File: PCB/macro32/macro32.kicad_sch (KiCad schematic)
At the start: 14 parts, among them J1 OLED, J2 OLED, J3 Magnetic connector, J4 Magnetic connector, J5 Magnetic connector, J6 Magnetic connector, SW1 RST, U1 SuperMini_NRF52840

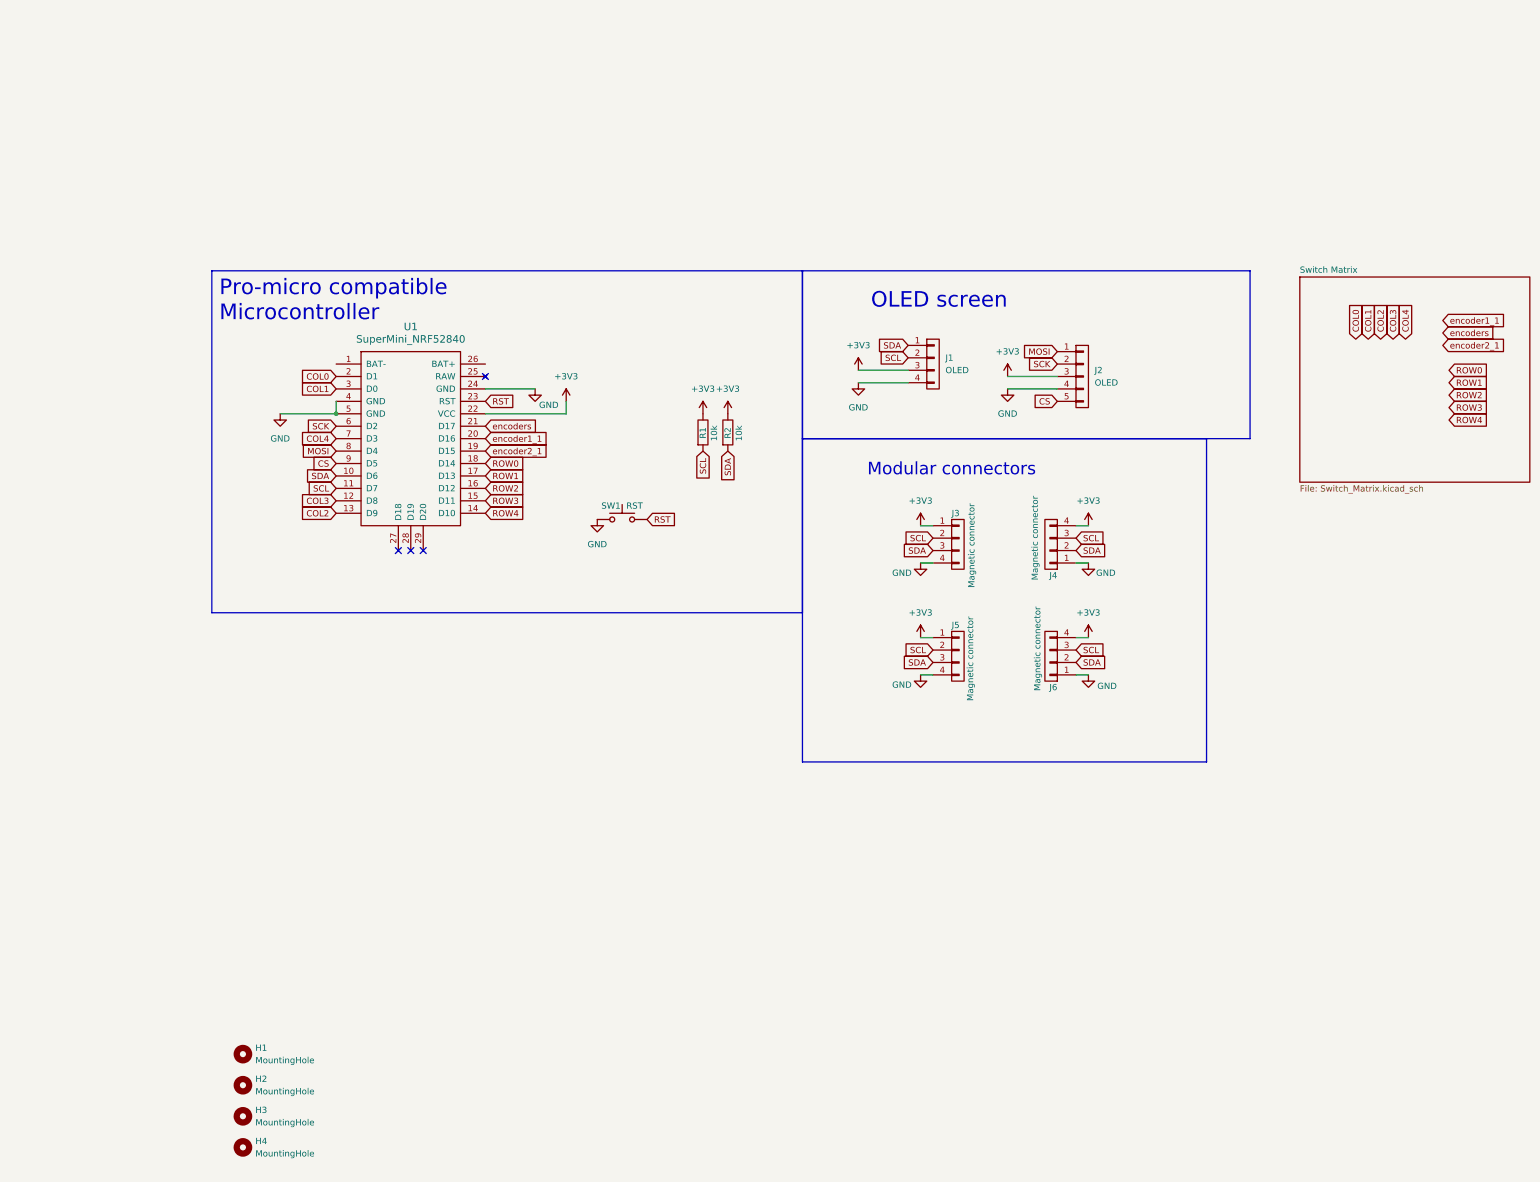
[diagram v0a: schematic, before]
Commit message: macro32_v2_schem&pcb
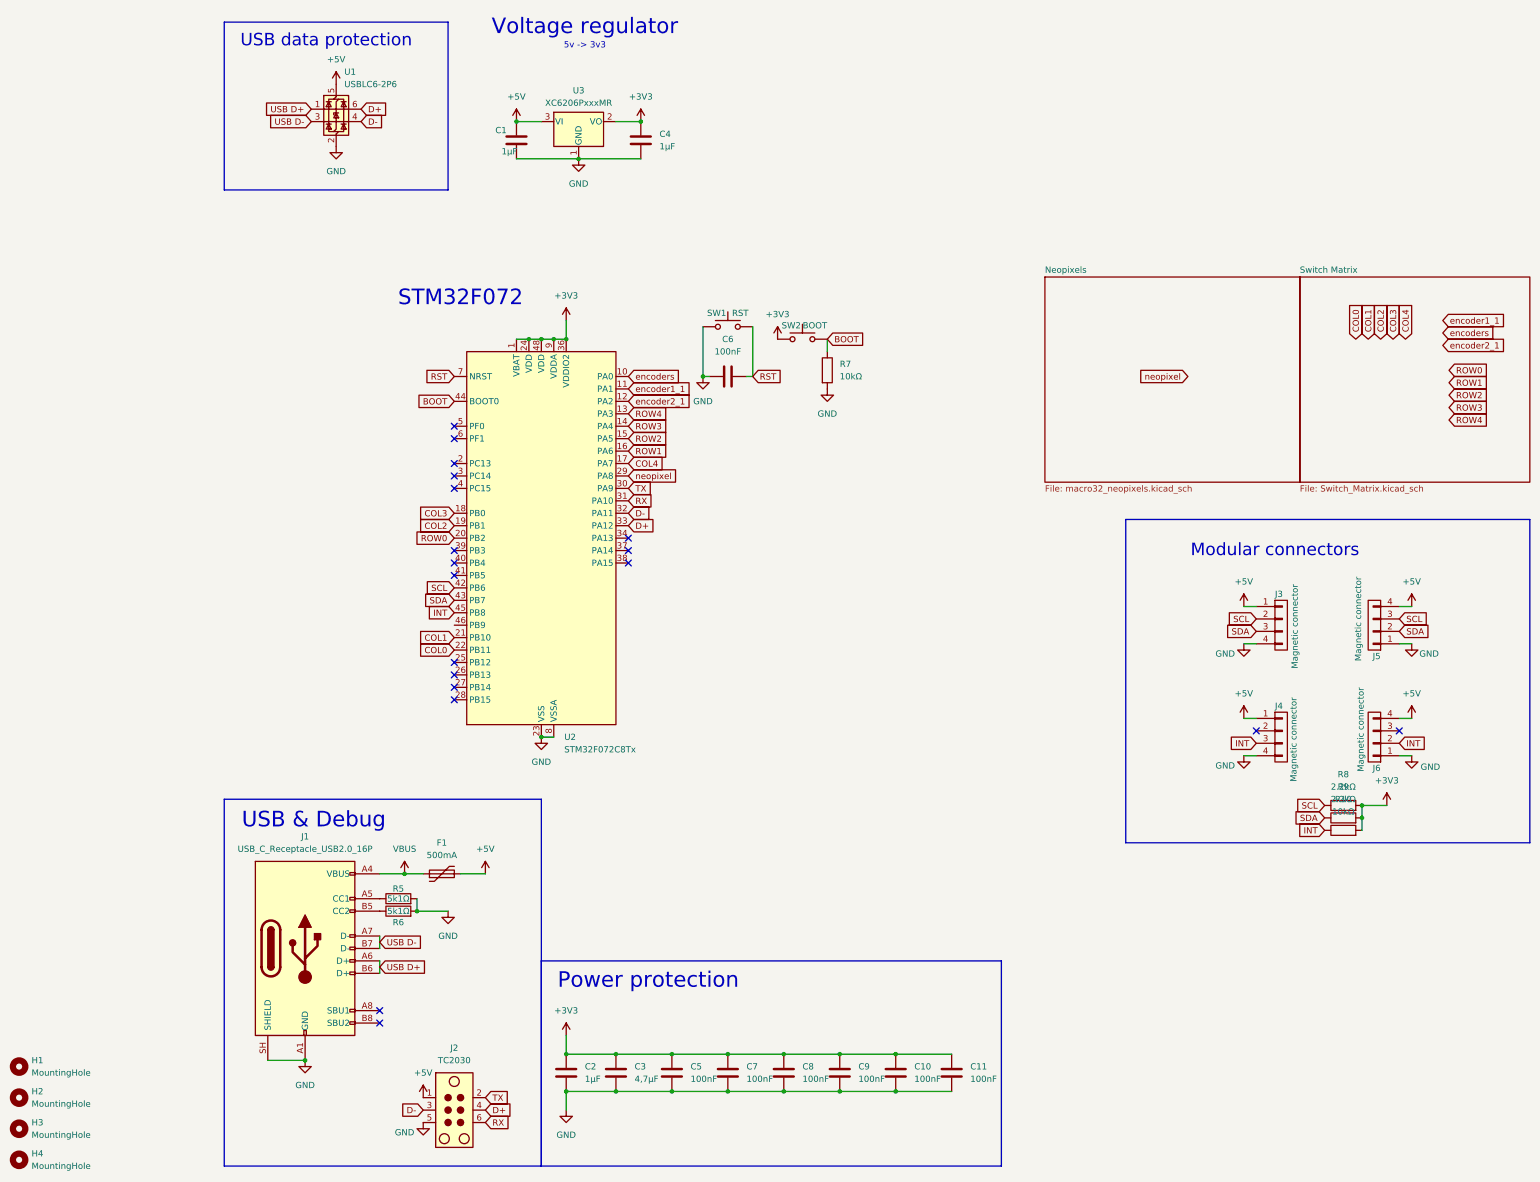
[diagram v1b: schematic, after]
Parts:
- removed J1: OLED, KillrOfLife_Connectors:OLED_4Pin, symbol KillrOfLife:OLED-4pin
- removed J2: OLED, KillrOfLife_Connectors:OLED_5Pin, symbol KillrOfLife:OLED-5pin
- removed R1, R2: 10k, Resistor_SMD:R_0805_2012Metric_Pad1.20x1.40mm_HandSolder, symbol Device:R
- removed U1: SuperMini_NRF52840, KillrOfLife_MCU:SuperMini_NRF52850_pro_micro, symbol ScottoKeebs:MCU_SuperMini_NRF52840
- added C1, C2, C4: 1μF, Capacitor_SMD:C_0805_2012Metric_Pad1.18x1.45mm_HandSolder, symbol Device:C
- added C10, C11, C5, C6, C7, C8, C9: 100nF, Capacitor_SMD:C_0805_2012Metric_Pad1.18x1.45mm_HandSolder, symbol Device:C
- added C3: 4,7μF, Capacitor_SMD:C_0805_2012Metric_Pad1.18x1.45mm_HandSolder, symbol Device:C
- added F1: 500mA, KillrOfLife_Components:Resistor_1206, symbol Device:Polyfuse
- added J1: USB_C_Receptacle_USB2.0_16P, Connector_USB:USB_C_Receptacle_GCT_USB4110, symbol Connector:USB_C_Receptacle_USB2.0_16P
- added J2: TC2030, Connector:Tag-Connect_TC2030-IDC-FP_2x03_P1.27mm_Vertical, symbol Connector:TC2030
- added R10, R7: 10kΩ, KillrOfLife_Components:Resistor_0805, symbol Device:R
- added R5, R6: 5k1Ω, KillrOfLife_Components:Resistor_0805, symbol Device:R
- added R8, R9: 2.2kΩ, KillrOfLife_Components:Resistor_0805, symbol Device:R
- added SW2: BOOT, Button_Switch_SMD:SW_SPST_TS-1088-xR020, symbol Switch:SW_Push
- added U1: USBLC6-2P6, Package_TO_SOT_SMD:SOT-666, symbol Power_Protection:USBLC6-2P6
- added U2: STM32F072C8Tx, Package_QFP:LQFP-48_7x7mm_P0.5mm, symbol MCU_ST_STM32F0:STM32F072C8Tx
- added U3: XC6206PxxxMR, Package_TO_SOT_SMD:SOT-23-3, symbol Regulator_Linear:XC6206PxxxMR
- J3: footprint Library:fakemag4pin90degFemale -> KillrOfLife_Connectors:fakemag4pin90degFemale
- J4: renamed from J5; footprint Library:fakemag4pin90degFemale -> KillrOfLife_Connectors:fakemag4pin90degFemale
- J5: renamed from J4; footprint Library:fakemag4pin90degMale -> KillrOfLife_Connectors:fakemag4pin90degFemale
- J6: footprint Library:fakemag4pin90degMale -> KillrOfLife_Connectors:fakemag4pin90degFemale
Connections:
- net +3V3: now also C10.1, C11.1, C2.1, C3.1, C4.1, C5.1, C7.1, C8.1, C9.1, R10.2, R8.2, R9.2, SW2.1, U2.1 (VBAT), U2.24 (VDD), U2.36 (VDDIO2), U2.48 (VDD), U2.9 (VDDA), U3.2 (VO); no longer J3.1 (P1), J4.1 (P1), J5.4 (P4), J6.4 (P4)
- net COL0: now also U2.22 (PB11)
- net COL1: now also U2.21 (PB10)
- net COL2: now also U2.19 (PB1)
- net COL3: now also U2.18 (PB0)
- net COL4: now also U2.17 (PA7)
- net GND: now also C1.2, C10.2, C11.2, C2.2, C3.2, C4.2, C5.2, C6.1, C7.2, C8.2, C9.2, J1.A1 (GND), J1.A12 (GND), J1.B1 (GND), J1.B12 (GND), J1.SH (SHIELD), J2.5, R5.2, R6.2, R7.2, U1.2 (GND), U2.23 (VSS), U2.35 (VSS), U2.47 (VSS), U2.8 (VSSA), U3.1 (GND)
- net ROW0: now also U2.20 (PB2)
- net ROW1: now also U2.16 (PA6)
- net ROW2: now also U2.15 (PA5)
- net ROW3: now also U2.14 (PA4)
- net ROW4: now also U2.13 (PA3)
- net RST: now also C6.2, U2.7 (NRST)
- net SCL: now also R8.1, U2.42 (PB6); no longer J4.2 (P2), J6.3 (P3)
- net SDA: now also R9.1, U2.43 (PB7); no longer J4.3 (P3), J6.2 (P2)
- net encoder1_1: now also U2.11 (PA1)
- net encoder2_1: now also U2.12 (PA2)
- net encoders: now also U2.10 (PA0)
- new net: J1.B5 (CC2), R6.1
- new net: J1.A5 (CC1), R5.1
- new net +5V: C1.1, F1.2, J2.1, J3.1 (P1), J4.1 (P1), J5.4 (P4), J6.4 (P4), U1.5 (VBUS), U3.3 (VI)
- new net BOOT: R7.1, SW2.2, U2.44 (BOOT0)
- new net D+: J2.4, U1.6 (I/O1), U2.33 (PA12)
- new net D-: J2.3, U1.4 (I/O2), U2.32 (PA11)
- new net INT: J4.3 (P3), J6.2 (P2), R10.1, U2.45 (PB8)
- new net RX: J2.6, U2.31 (PA10)
- new net TX: J2.2, U2.30 (PA9)
- new net USB D+: J1.A6 (D+), J1.B6 (D+), U1.1 (I/O1)
- new net USB D-: J1.A7 (D-), J1.B7 (D-), U1.3 (I/O2)
- new net VBUS: F1.1, J1.A4 (VBUS), J1.A9 (VBUS), J1.B4 (VBUS), J1.B9 (VBUS)
- new net neopixel: U2.29 (PA8)
- no-connect marks 4 -> 19
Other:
- added sheet Neopixels (macro32_neopixels.kicad_sch)
- note added: "5v -> 3v3"
- note added: "Power protection"
- note added: "STM32F072"
- note added: "USB & Debug"
- note added: "USB data protection"
- note added: "Voltage regulator"
- note removed: "OLED screen"
- note removed: "Pro-micro compatible Microcontroller"
- moved on the sheet: H1, H2, H3, H4, J3, J4, J5, J6
